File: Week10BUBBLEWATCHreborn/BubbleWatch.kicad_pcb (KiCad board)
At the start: 2 copper layers, 84 x 38 mm, 38 parts, among them J1 Conn_02x02_Counter_Clockwise, J2 Conn_02x02_Counter_Clockwise, J3 Conn_01x05, SW1 SW_Push, SW2 SW_Push, SW3 SW_Push, SW4 SW_Push, U1 RedRetroBubbleDisplay, U2 RedRetroBubbleDisplay, U3 STM32F030C8Tx, U4 MCP1640BCH, Y1 Crystal

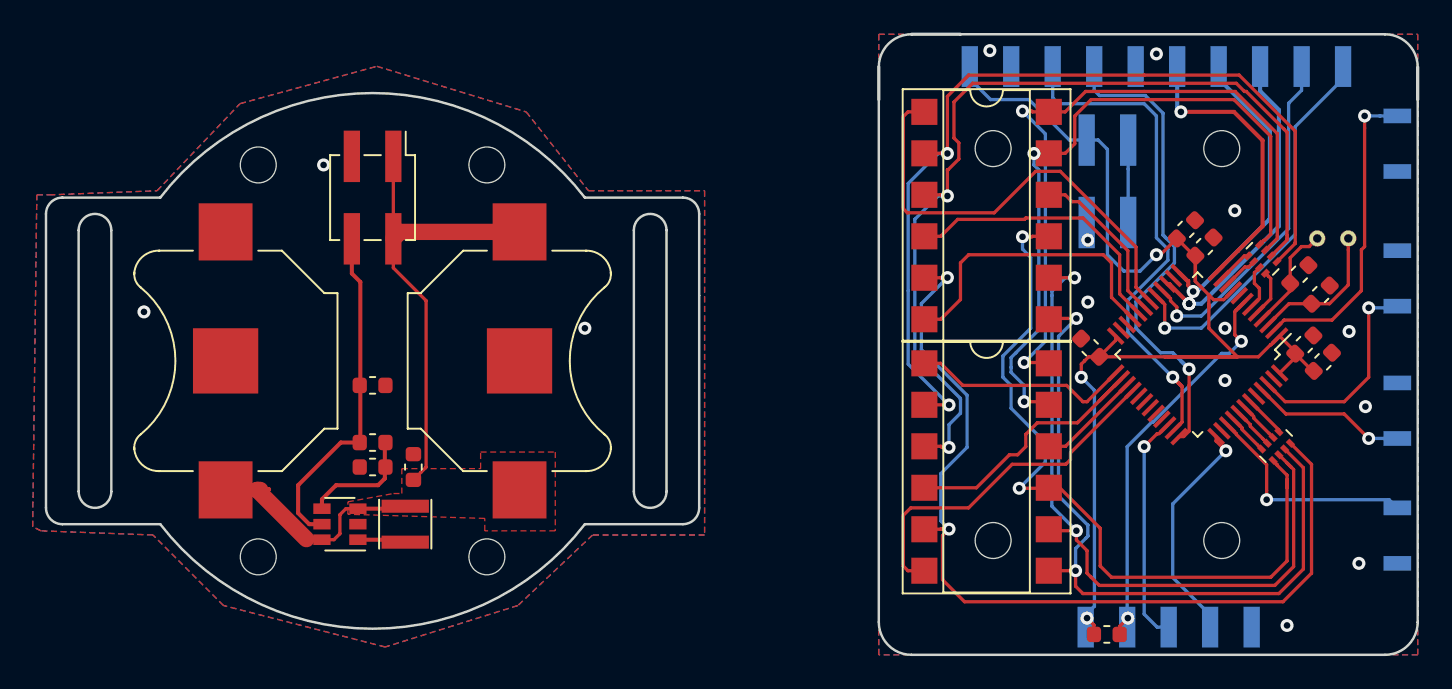
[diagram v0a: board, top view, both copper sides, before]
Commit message: Rain silks and gerber done
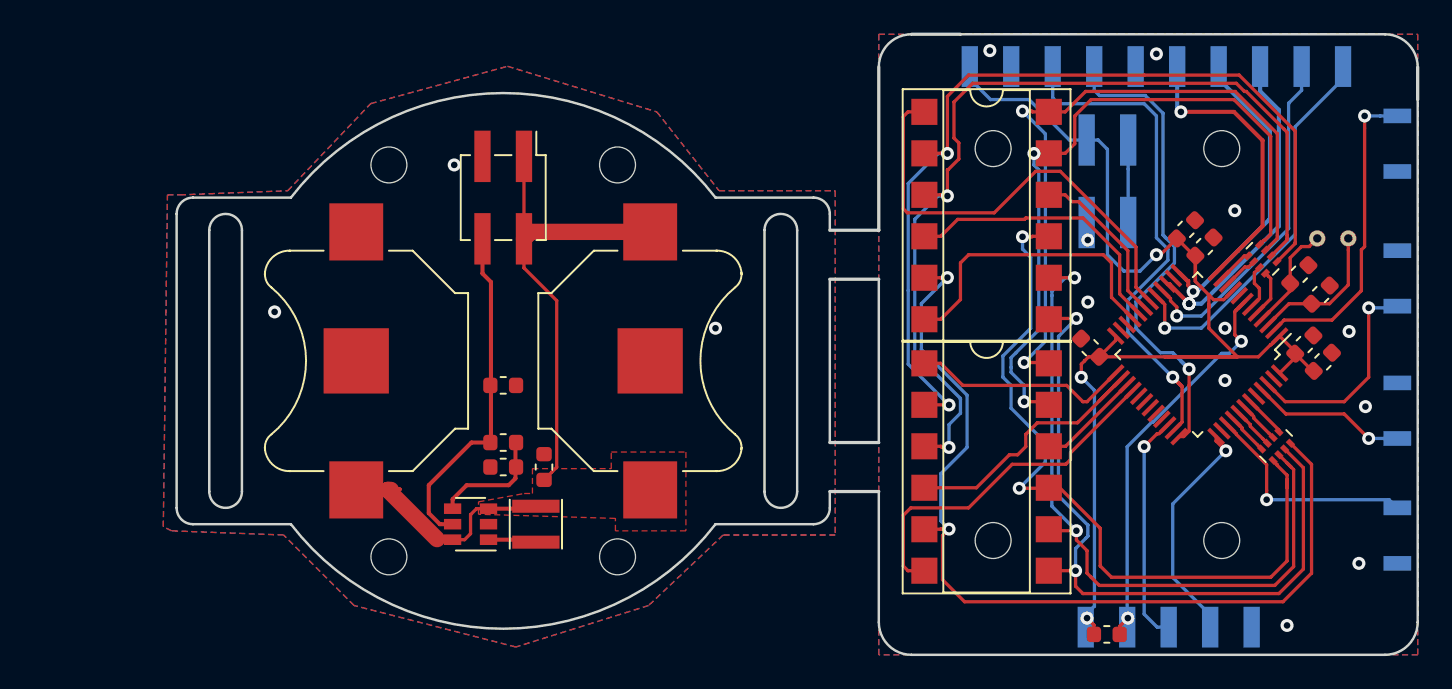
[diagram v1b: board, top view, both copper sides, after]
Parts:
- moved BT1 8.00 mm to (113.0, 79.0)
- moved BT2 8.00 mm to (95.0, 79.0)
- moved C7 8.00 mm to (106.5, 85.5)
- moved C9 8.00 mm to (104.0, 80.5)
- moved J1 8.00 mm to (104.0, 69.0)
- moved L1 8.00 mm to (106.0, 89.0)
- moved R1 8.00 mm to (104.0, 84.0)
- moved R2 8.00 mm to (104.0, 85.5)
- moved REF** 8.00 mm to (97.0, 67.0)
- moved REF** 8.00 mm to (111.0, 67.0)
- moved REF** 8.00 mm to (111.0, 91.0)
- moved REF** 8.00 mm to (97.0, 91.0)
- moved U4 8.00 mm to (102.0, 89.0)
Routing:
- net GND: vias 14 -> 13
- net (no net): vias 4 -> 5
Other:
- board size 84 x 38 mm -> 76 x 38 mm
